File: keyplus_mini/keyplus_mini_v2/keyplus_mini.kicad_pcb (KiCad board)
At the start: 2 copper layers, 24 x 23 mm, 22 parts, among them J1 USB_TYPE_C, J2 Conn_02x09_Odd_Even, J3 CONN_01X01, J4 Conn_02x09_Odd_Even, U1 MCP1700-3302E_SOT23, U2 ATXMEGA16A4U-MH_EPAD

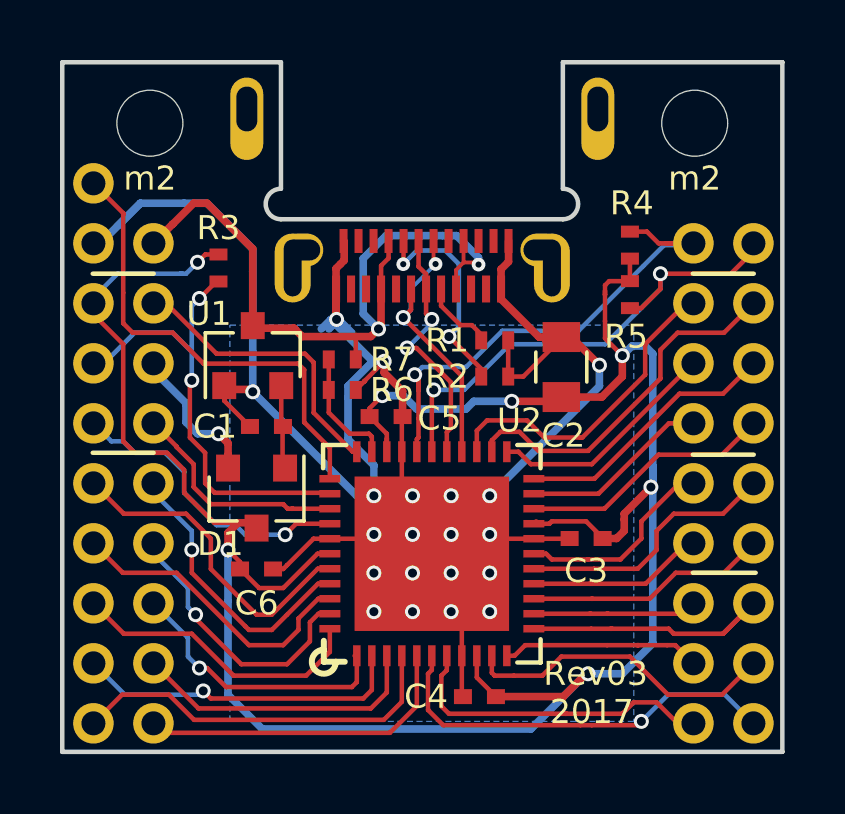
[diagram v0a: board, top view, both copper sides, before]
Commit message: clean up libraries
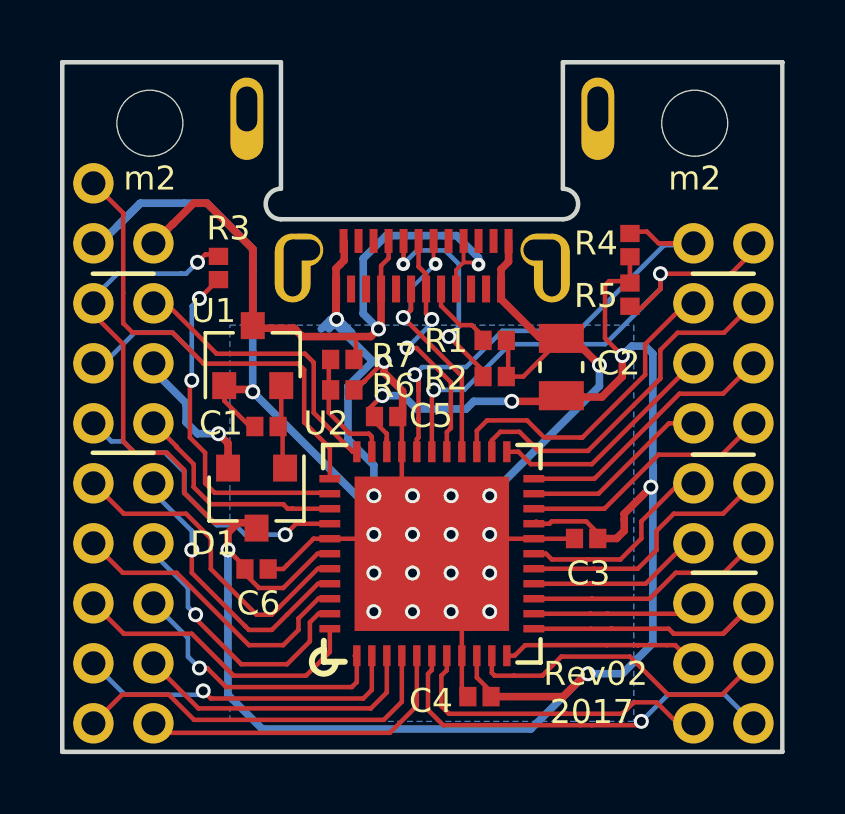
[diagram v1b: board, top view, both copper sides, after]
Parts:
- C1, C3, C4, C5, C6: footprint Capacitors_SMD:C_0402_NoSilk -> Capacitor_SMD:C_0402_1005Metric
- C2: footprint Capacitors_SMD:C_0805 -> Capacitor_SMD:C_0805_2012Metric
- D1, U1: footprint TO_SOT_Packages_SMD:SOT-23 -> Package_TO_SOT_SMD:SOT-23
- J1: footprint connectors:DX07B024JJ1R1300 -> conn_usb:DX07B024JJ1R1300
- J2, J4: footprint headers:Pin_Header_Straight_2x09_Pitch2.00mm_No_Silk -> Conn_PinHeader_2.00mm:PinHeader_2x09_P2.00mm_Vertical
- J3: footprint headers:Pin_Header_Straight_1x01_Pitch2.00mm_No_Silk -> Conn_PinHeader_2.00mm:PinHeader_1x01_P2.00mm_Vertical
- R1, R2, R3, R4, R5, R6, R7: footprint Resistors_SMD:R_0402_NoSilk -> Resistor_SMD:R_0402_1005Metric
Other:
- board text added: "Rev02"
- board text removed: "Rev03"
